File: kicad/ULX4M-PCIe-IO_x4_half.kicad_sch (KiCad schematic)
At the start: 99 parts, among them J10 FCR684205R, J11 OLED, J12 641737-1, J13 39-30-0060, J14 LM7805_EN, J15 POE, J16 Barrel_Jack, J17 JTAG, J18 I2C_to_ID, J19 PCIe_JTAG, J20 PCIe_I2C, J21 PCIe_1X_4X, J3 SFP+, J4 SFP+, J5 HAT, J6 EXT_USB, J7 Micro_SD_Card_CD, J8 Board_To_Board, J9 FCR684205T, SW1 SW_DIP_x08, SW2 SW_DIP_x08, U10 TPD4E02B04DQA, U11 TPD4E02B04DQA, U12 TPD4E02B04DQA, U13 AT24CS32-SSHM, U14 LM78M05_TO252, U9 TPD4E02B04DQA

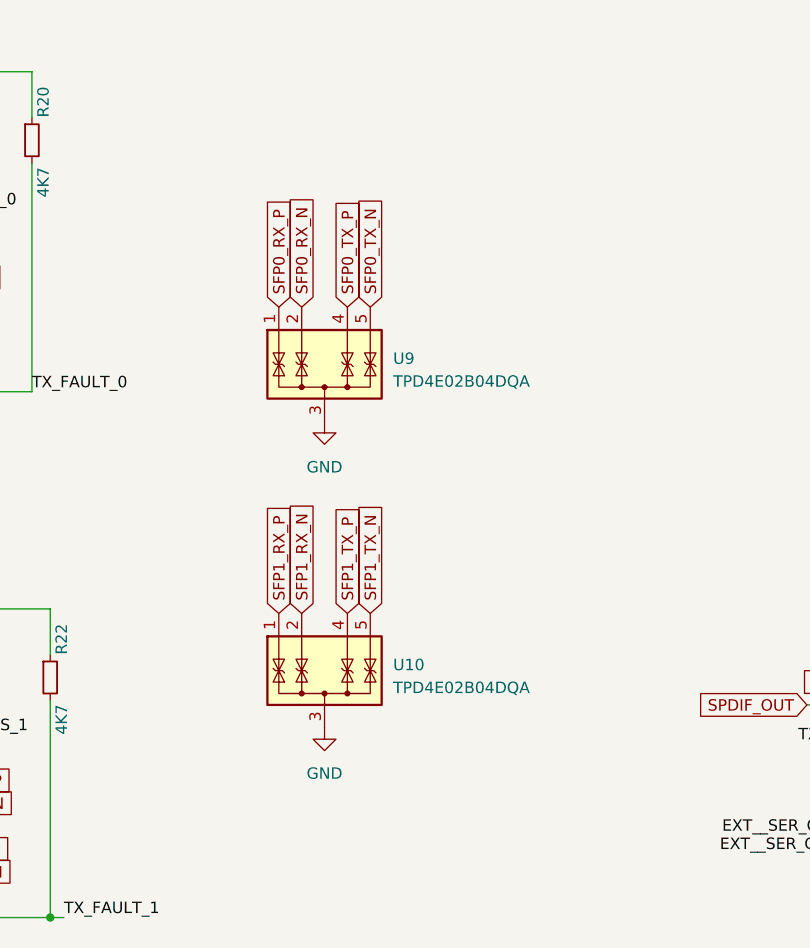
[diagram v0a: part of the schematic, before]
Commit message: Routing
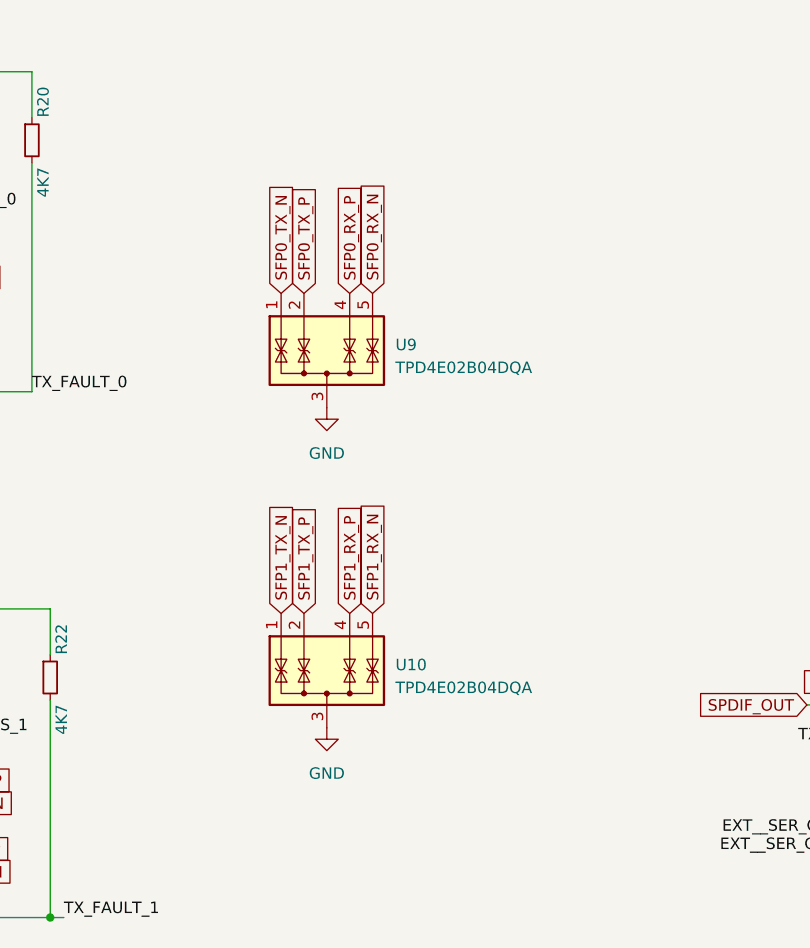
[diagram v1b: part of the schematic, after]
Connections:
- net SFP0_RX_N: now also U9.5 (IO4); no longer U9.2 (IO2)
- net SFP0_RX_P: now also U9.4 (IO3); no longer U9.1 (IO1)
- net SFP0_TX_N: now also U9.1 (IO1); no longer U9.5 (IO4)
- net SFP0_TX_P: now also U9.2 (IO2); no longer U9.4 (IO3)
- net SFP1_RX_N: now also U10.5 (IO4); no longer U10.2 (IO2)
- net SFP1_RX_P: now also U10.4 (IO3); no longer U10.1 (IO1)
- net SFP1_TX_N: now also U10.1 (IO1); no longer U10.5 (IO4)
- net SFP1_TX_P: now also U10.2 (IO2); no longer U10.4 (IO3)
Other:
- moved on the sheet: U9
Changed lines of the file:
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@@
     )
   )
-  (global_label "SFP0_TX_N" (shape input) (at 1.016 -98.806 90) (fields_autoplaced)
+  (global_label "SFP0_TX_N" (shape input) (at -8.89 -100.33 90) (fields_autoplaced)
     (effects (font (size 1.27 1.27)) (justify left))
-    (property "Intersheetrefs" "${INTERSHEET_REFS}" (at 2.8512 -98.806 90)
+    (property "Intersheetrefs" "${INTERSHEET_REFS}" (at -7.0548 -100.33 90)
       (effects (font (size 1.27 1.27)) (justify left) hide)
     )
@@
     )
   )
-  (global_label "SFP0_TX_P" (shape input) (at -1.524 -98.806 90) (fields_autoplaced)
+  (global_label "SFP0_TX_P" (shape input) (at -6.35 -100.33 90) (fields_autoplaced)
     (effects (font (size 1.27 1.27)) (justify left))
-    (property "Intersheetrefs" "${INTERSHEET_REFS}" (at 0.3112 -98.806 90)
+    (property "Intersheetrefs" "${INTERSHEET_REFS}" (at -4.5148 -100.33 90)
       (effects (font (size 1.27 1.27)) (justify left) hide)
     )
@@
     )
   )
-  (global_label "SFP1_TX_N" (shape input) (at 1.016 -64.77 90) (fields_autoplaced)
+  (global_label "SFP1_TX_N" (shape input) (at -8.89 -64.77 90) (fields_autoplaced)
     (effects (font (size 1.27 1.27)) (justify left))
-    (property "Intersheetrefs" "${INTERSHEET_REFS}" (at 2.8512 -64.77 90)
+    (property "Intersheetrefs" "${INTERSHEET_REFS}" (at -7.0548 -64.77 90)
       (effects (font (size 1.27 1.27)) (justify left) hide)
     )
@@
     )
   )
-  (global_label "SFP1_TX_P" (shape input) (at -1.524 -64.77 90) (fields_autoplaced)
+  (global_label "SFP1_TX_P" (shape input) (at -6.35 -64.77 90) (fields_autoplaced)
     (effects (font (size 1.27 1.27)) (justify left))
-    (property "Intersheetrefs" "${INTERSHEET_REFS}" (at 0.3112 -64.77 90)
+    (property "Intersheetrefs" "${INTERSHEET_REFS}" (at -4.5148 -64.77 90)
       (effects (font (size 1.27 1.27)) (justify left) hide)
     )
@@
     )
   )
-  (global_label "SFP0_RX_P" (shape input) (at -9.144 -98.806 90) (fields_autoplaced)
+  (global_label "SFP0_RX_P" (shape input) (at -1.27 -100.33 90) (fields_autoplaced)
     (effects (font (size 1.27 1.27)) (justify left))
-    (property "Intersheetrefs" "${INTERSHEET_REFS}" (at -7.3088 -98.806 90)
+    (property "Intersheetrefs" "${INTERSHEET_REFS}" (at 0.5652 -100.33 90)
       (effects (font (size 1.27 1.27)) (justify left) hide)
     )
@@
     )
   )
-  (global_label "SFP1_RX_P" (shape input) (at -9.144 -64.77 90) (fields_autoplaced)
+  (global_label "SFP1_RX_P" (shape input) (at -1.27 -64.77 90) (fields_autoplaced)
     (effects (font (size 1.27 1.27)) (justify left))
-    (property "Intersheetrefs" "${INTERSHEET_REFS}" (at -7.3088 -64.77 90)
+    (property "Intersheetrefs" "${INTERSHEET_REFS}" (at 0.5652 -64.77 90)
       (effects (font (size 1.27 1.27)) (justify left) hide)
     )
@@
     )
   )
-  (global_label "SFP0_RX_N" (shape input) (at -6.604 -98.806 90) (fields_autoplaced)
+  (global_label "SFP0_RX_N" (shape input) (at 1.27 -100.33 90) (fields_autoplaced)
     (effects (font (size 1.27 1.27)) (justify left))
-    (property "Intersheetrefs" "${INTERSHEET_REFS}" (at -4.7688 -98.806 90)
+    (property "Intersheetrefs" "${INTERSHEET_REFS}" (at 3.1052 -100.33 90)
       (effects (font (size 1.27 1.27)) (justify left) hide)
     )
@@
     )
   )
-  (global_label "SFP1_RX_N" (shape input) (at -6.604 -64.77 90) (fields_autoplaced)
+  (global_label "SFP1_RX_N" (shape input) (at 1.27 -64.77 90) (fields_autoplaced)
     (effects (font (size 1.27 1.27)) (justify left))
-    (property "Intersheetrefs" "${INTERSHEET_REFS}" (at -4.7688 -64.77 90)
+    (property "Intersheetrefs" "${INTERSHEET_REFS}" (at 3.1052 -64.77 90)
       (effects (font (size 1.27 1.27)) (justify left) hide)
     )
@@
   (symbol (lib_id "power:GND") (at 21.59 195.58 0) (unit 1)
     (in_bom yes) (on_board yes) (dnp no) (fields_autoplaced)
-    (property "Reference" "#PWR0154" (at 21.59 201.93 0)
+    (property "Reference" "#PWR0281" (at 21.59 201.93 0)
       (effects (font (size 1.27 1.27)) hide)
     )
@@
       (project "ULX4M-PCIe-IO_x4_half"
         (path "/e227bafe-08dc-4b2a-9df8-340d24e6faf1"
-          (reference "#PWR0154") (unit 1) (value "GND") (footprint "")
+          (reference "#PWR0281") (unit 1) (value "GND") (footprint "")
         )
       )
@@
     )
   )
-  (symbol (lib_id "power:GND") (at -4.064 -52.07 0) (unit 1)
+  (symbol (lib_id "power:GND") (at -3.81 -52.07 0) (unit 1)
     (in_bom yes) (on_board yes) (dnp no) (fields_autoplaced)
-    (property "Reference" "#PWR0229" (at -4.064 -45.72 0)
+    (property "Reference" "#PWR0229" (at -3.81 -45.72 0)
       (effects (font (size 1.27 1.27)) hide)
     )
-    (property "Value" "GND" (at -4.064 -46.99 0)
+    (property "Value" "GND" (at -3.81 -46.99 0)
       (effects (font (size 1.27 1.27)))
     )
-    (property "Footprint" "" (at -4.064 -52.07 0)
+    (property "Footprint" "" (at -3.81 -52.07 0)
       (effects (font (size 1.27 1.27)) hide)
     )
-    (property "Datasheet" "" (at -4.064 -52.07 0)
+    (property "Datasheet" "" (at -3.81 -52.07 0)
       (effects (font (size 1.27 1.27)) hide)
     )
@@
     )
   )
-  (symbol (lib_id "power:GND") (at -4.064 -86.106 0) (unit 1)
+  (symbol (lib_id "power:GND") (at -3.81 -87.63 0) (unit 1)
     (in_bom yes) (on_board yes) (dnp no) (fields_autoplaced)
-    (property "Reference" "#PWR0230" (at -4.064 -79.756 0)
+    (property "Reference" "#PWR0230" (at -3.81 -81.28 0)
       (effects (font (size 1.27 1.27)) hide)
     )
-    (property "Value" "GND" (at -4.064 -81.026 0)
+    (property "Value" "GND" (at -3.81 -82.55 0)
       (effects (font (size 1.27 1.27)))
     )
-    (property "Footprint" "" (at -4.064 -86.106 0)
+    (property "Footprint" "" (at -3.81 -87.63 0)
       (effects (font (size 1.27 1.27)) hide)
     )
-    (property "Datasheet" "" (at -4.064 -86.106 0)
+    (property "Datasheet" "" (at -3.81 -87.63 0)
       (effects (font (size 1.27 1.27)) hide)
     )
@@
     )
   )
-  (symbol (lib_id "Power_Protection:TPD4E02B04DQA") (at -4.064 -57.15 0) (unit 1)
+  (symbol (lib_id "Power_Protection:TPD4E02B04DQA") (at -3.81 -57.15 0) (unit 1)
     (in_bom yes) (on_board yes) (dnp no) (fields_autoplaced)
-    (property "Reference" "U10" (at 3.556 -59.055 0)
+    (property "Reference" "U10" (at 3.81 -59.055 0)
       (effects (font (size 1.27 1.27)) (justify left))
     )
-    (property "Value" "TPD4E02B04DQA" (at 3.556 -56.515 0)
+    (property "Value" "TPD4E02B04DQA" (at 3.81 -56.515 0)
       (effects (font (size 1.27 1.27)) (justify left))
     )
-    (property "Footprint" "Package_SON:USON-10_2.5x1.0mm_P0.5mm" (at 3.556 -57.15 0)
+    (property "Footprint" "Package_SON:USON-10_2.5x1.0mm_P0.5mm" (at 3.81 -57.15 0)
       (effects (font (size 1.27 1.27)) (justify left) hide)
     )
-    (property "Datasheet" "http://www.ti.com/lit/ds/symlink/tpd4e02b04.pdf" (at -0.889 -65.405 0)
+    (property "Datasheet" "http://www.ti.com/lit/ds/symlink/tpd4e02b04.pdf" (at -0.635 -65.405 0)
       (effects (font (size 1.27 1.27)) hide)
     )
@@
   (symbol (lib_id "power:GND") (at 31.75 142.24 180) (unit 1)
     (in_bom yes) (on_board yes) (dnp no) (fields_autoplaced)
-    (property "Reference" "#PWR0154" (at 31.75 135.89 0)
+    (property "Reference" "#PWR0282" (at 31.75 135.89 0)
       (effects (font (size 1.27 1.27)) hide)
     )
@@
       (project "ULX4M-PCIe-IO_x4_half"
         (path "/e227bafe-08dc-4b2a-9df8-340d24e6faf1"
-          (reference "#PWR0154") (unit 1) (value "GND") (footprint "")
+          (reference "#PWR0282") (unit 1) (value "GND") (footprint "")
         )
       )
@@
     )
   )
-  (symbol (lib_id "Power_Protection:TPD4E02B04DQA") (at -4.064 -91.186 0) (unit 1)
+  (symbol (lib_id "Power_Protection:TPD4E02B04DQA") (at -3.81 -92.71 0) (unit 1)
     (in_bom yes) (on_board yes) (dnp no) (fields_autoplaced)
-    (property "Reference" "U9" (at 3.556 -93.091 0)
+    (property "Reference" "U9" (at 3.81 -94.615 0)
       (effects (font (size 1.27 1.27)) (justify left))
     )
-    (property "Value" "TPD4E02B04DQA" (at 3.556 -90.551 0)
+    (property "Value" "TPD4E02B04DQA" (at 3.81 -92.075 0)
       (effects (font (size 1.27 1.27)) (justify left))
     )
-    (property "Footprint" "Package_SON:USON-10_2.5x1.0mm_P0.5mm" (at 3.556 -91.186 0)
+    (property "Footprint" "Package_SON:USON-10_2.5x1.0mm_P0.5mm" (at 3.81 -92.71 0)
       (effects (font (size 1.27 1.27)) (justify left) hide)
     )
-    (property "Datasheet" "http://www.ti.com/lit/ds/symlink/tpd4e02b04.pdf" (at -0.889 -99.441 0)
+    (property "Datasheet" "http://www.ti.com/lit/ds/symlink/tpd4e02b04.pdf" (at -0.635 -100.965 0)
       (effects (font (size 1.27 1.27)) hide)
     )

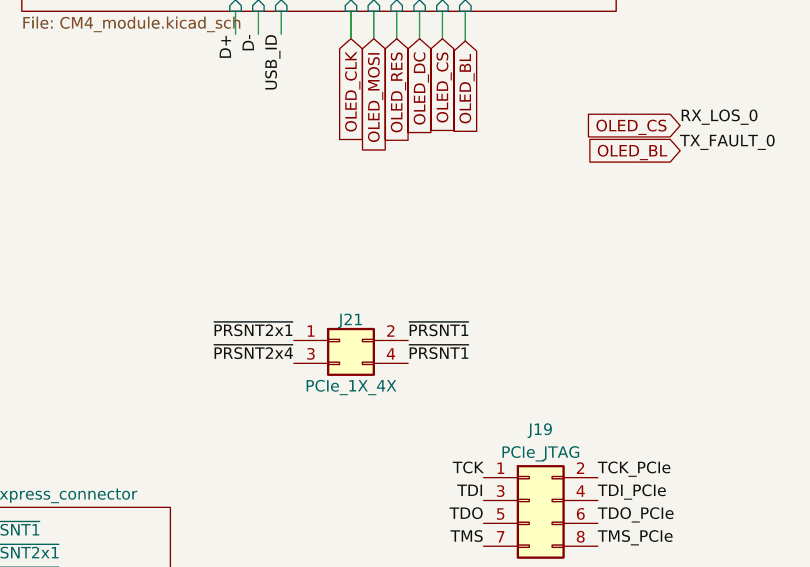
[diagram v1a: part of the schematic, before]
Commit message: Routing
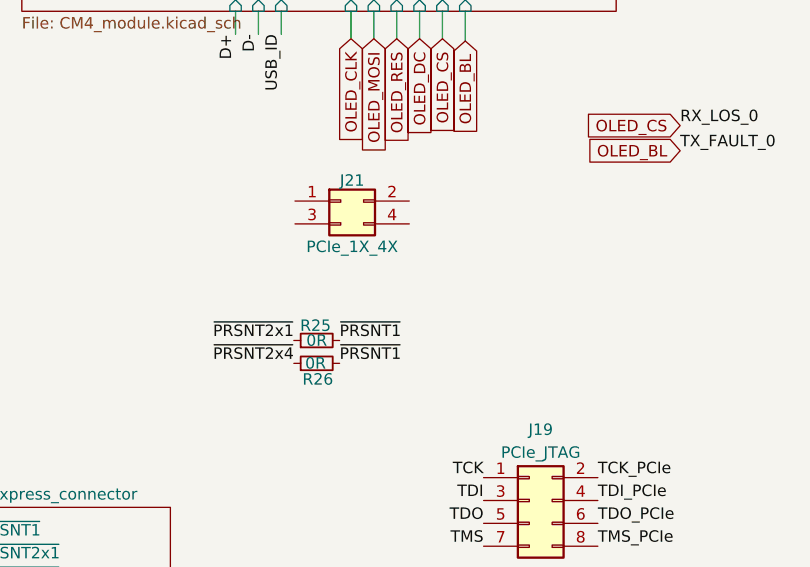
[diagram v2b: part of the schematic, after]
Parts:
- added R25, R26: 0R, symbol Device:R_Small
- J16: footprint CM4IO:BarrelJack_Horizontal -> Connector_BarrelJack:BarrelJack_Horizontal
- U10, U11, U12, U9: footprint Package_SON:USON-10_2.5x1.0mm_P0.5mm -> TPD4E02:USON-10_2.5x1.0mm_P0.5mm
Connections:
- net ~{PRSNT1}: now also R25.2, R26.2; no longer J21.2 (Pin_2), J21.4 (Pin_4)
- net ~{PRSNT2x1}: now also R25.1; no longer J21.1 (Pin_1)
- net ~{PRSNT2x4}: now also R26.1; no longer J21.3 (Pin_3)
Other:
- moved on the sheet: J21

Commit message: uređena schema
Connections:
- net ~{PRSNT1}: no longer R26.2
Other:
- note added: "${project_creator} License: ${project_license} Year: ${project_year}"
- note added: "${project_name}"
- note added: "......"
- note added: "11"
- note added: "2"
- note added: "CM4_module"
- note added: "Index"
- note added: "PCIexpress_connector"
- note added: "Page"
- company: Author: Luca Anastasio -> ${project_creator}
- title: PCIexpress_x4_half -> ${project_name} ${project_version}
- moved on the sheet: AE1, AE2, AE3, C10, C11, C12, C13, C14, C15, C9, D1, D10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
